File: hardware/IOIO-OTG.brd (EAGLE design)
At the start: 68.6 x 30.5 mm, 60 parts, among them Q1 IRLML2244, Q2 2N7002PW, Q3 AO3404A, U1 PIC24FJ256GB206, U14 SWITCH_SPDT, U2 TPS62133RGTT, U3 VREG_MIC5216

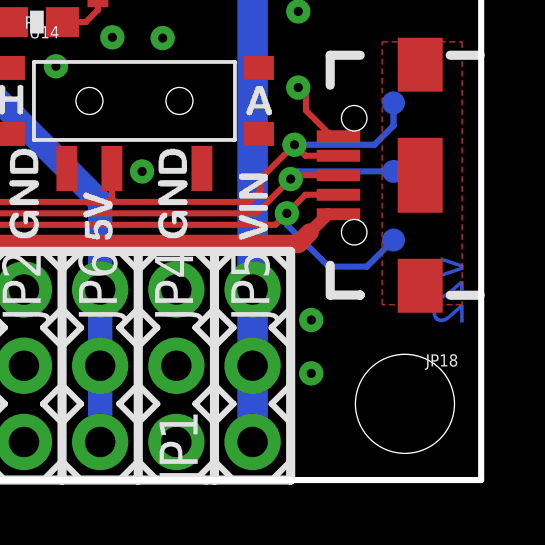
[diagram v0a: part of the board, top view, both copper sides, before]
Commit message: v22a in copper and sch
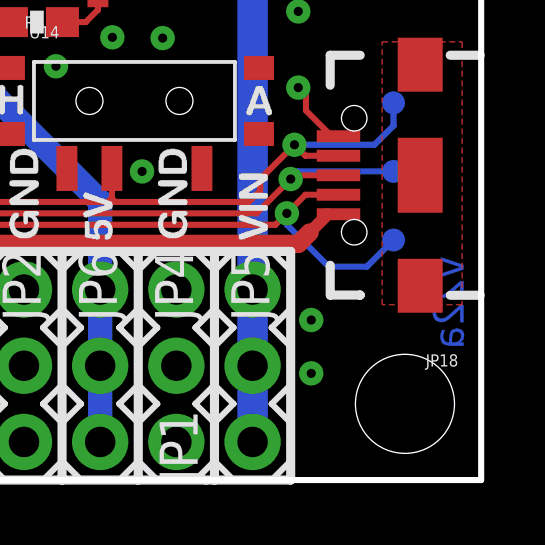
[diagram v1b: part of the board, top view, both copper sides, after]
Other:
- board text added: "v22a"
- board text removed: "v22"
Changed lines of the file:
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@@
 <circle x="55.88" y="29.21" radius="1.1039" width="0.508" layer="22"/>
 <circle x="53.34" y="29.21" radius="1.1039" width="0.508" layer="22"/>
-<text x="67.9958" y="7.4676" size="1.016" layer="16" font="vector" ratio="20" rot="SMR270">v22</text>
+<text x="67.9958" y="7.4676" size="1.016" layer="16" font="vector" ratio="20" rot="SMR270">v22a</text>
 <wire x1="57.15" y1="30.48" x2="59.69" y2="30.48" width="0.3048" layer="21"/>
 <wire x1="59.69" y1="27.94" x2="59.69" y2="30.48" width="0.3048" layer="21"/>
